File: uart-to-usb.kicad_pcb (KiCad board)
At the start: 2 copper layers, 43.5 x 29.5 mm, 9 parts, among them J1 USB_C_Receptacle_USB2.0_16P, U1 FT232RL

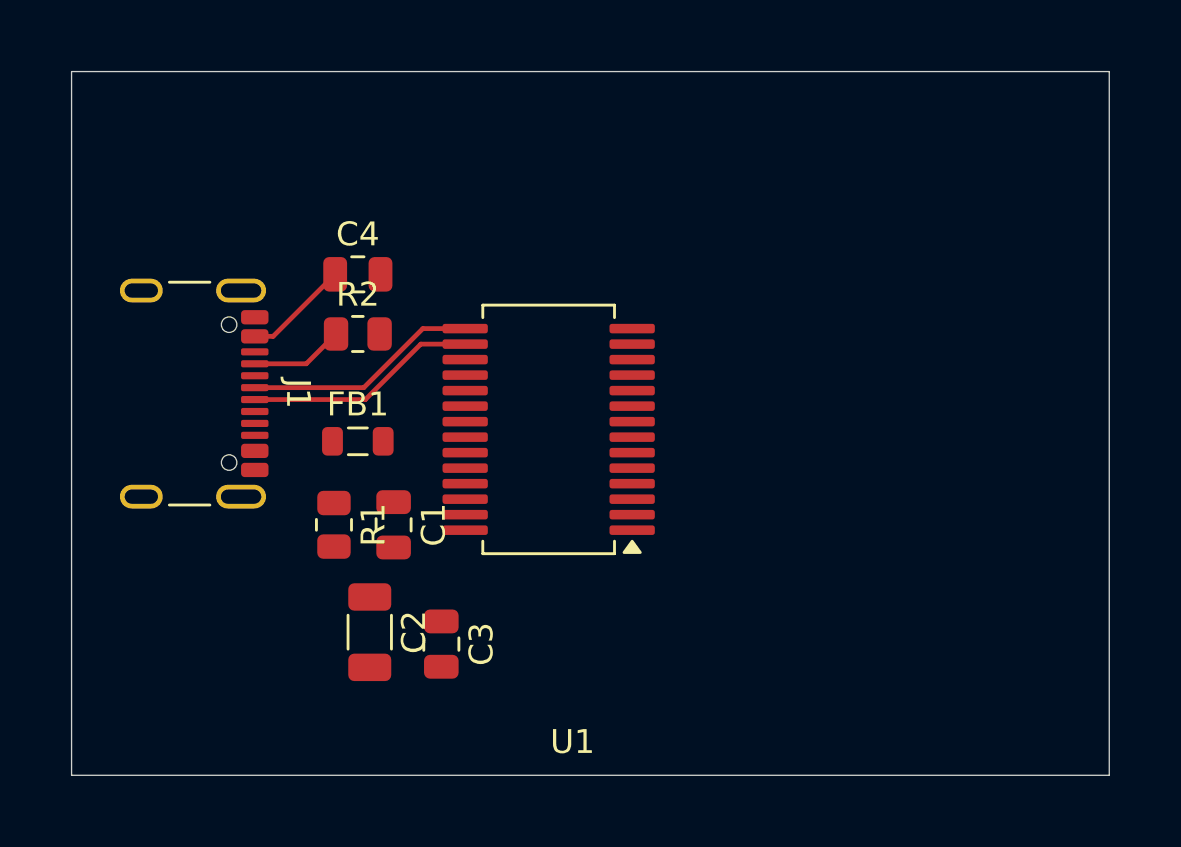
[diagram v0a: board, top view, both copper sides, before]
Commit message: Initial PCB route
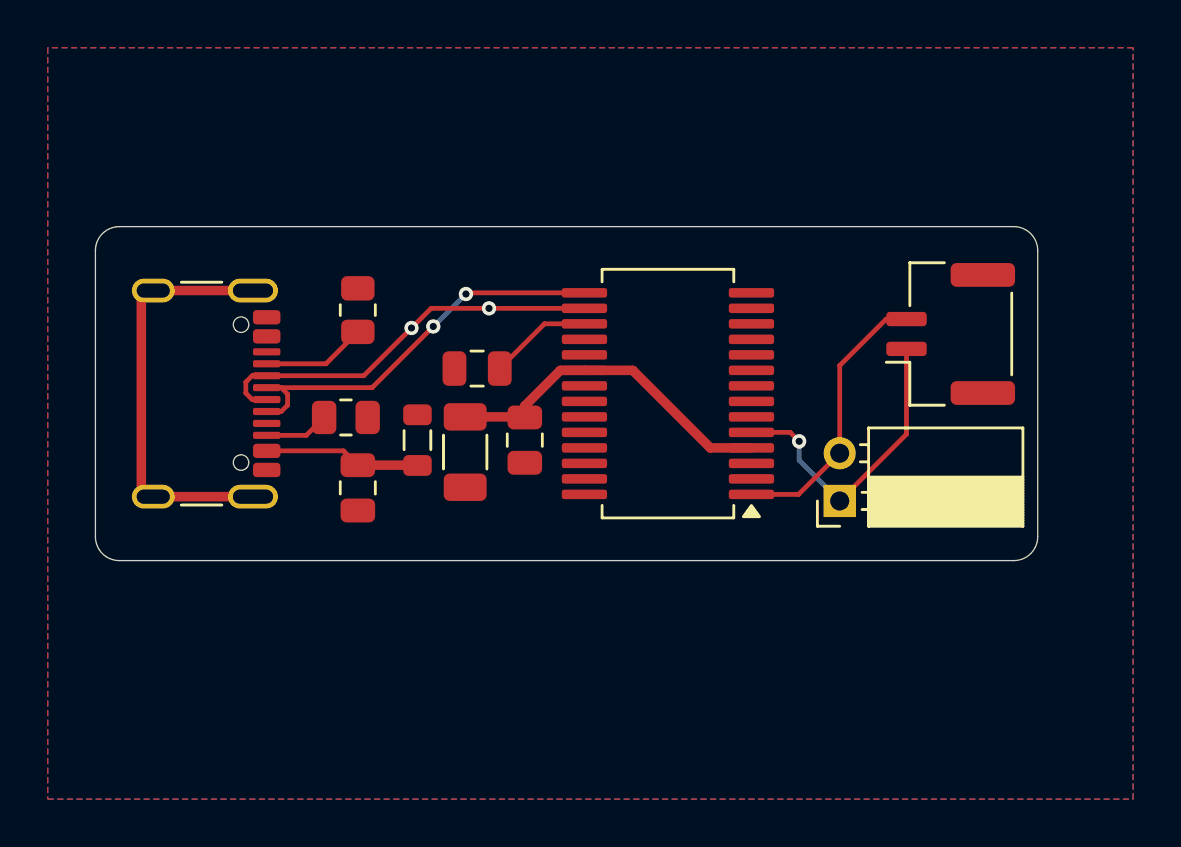
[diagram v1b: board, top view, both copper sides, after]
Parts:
- added J2: Conn_01x02_Pin, Connector_JST:JST_GH_SM02B-GHS-TB_1x02-1MP_P1.25mm_Horizontal, F.Cu at (159.8, 94.0)
- added J3: Conn_01x02_Pin, Connector_PinSocket_2.00mm:PinSocket_1x02_P2.00mm_Horizontal, F.Cu at (155.2, 101.0)
- moved C3 9.24 mm to (142.0, 98.5)
- moved C4 8.95 mm to (135.0, 100.5), turned to -90 degrees
- moved C2 8.54 mm to (139.5, 99.0)
- moved C1 7.43 mm to (140.0, 95.5), turned to 180 degrees
- moved U1 5.22 mm to (148.0, 96.5)
- moved R1 4.53 mm to (134.5, 97.5), turned to 0 degrees
- moved FB1 2.50 mm to (137.5, 98.5), turned to -90 degrees
- moved R2 1.00 mm to (135.0, 93.0), turned to 90 degrees
- moved J1 0.50 mm to (127.5, 96.5)
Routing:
- net unconnected-(J1-SHIELD-PadSH): track 0.00 -> 17.0 mm
- net +5V: track 0.00 -> 14.6 mm
- net Net-(J2-Pin_1): track 0.00 -> 12.9 mm, vias 0 -> 1
- net Net-(J2-Pin_2): track 0.00 -> 11.7 mm
- net /D+: track 9.85 -> 17.4 mm, vias 0 -> 2
- net /D-: track 9.78 -> 16.9 mm, vias 0 -> 2
- net Net-(U1-3V3OUT): track 0.00 -> 4.33 mm
- net Net-(J1-CC2): track 0.00 -> 2.72 mm
- net Net-(C4-Pad1): track 4.45 -> 6.07 mm
- added copper zone on B.Cu, net GND
- added copper zone on F.Cu, net GND
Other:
- board size 43.5 x 29.5 mm -> 39.5 x 14 mm
